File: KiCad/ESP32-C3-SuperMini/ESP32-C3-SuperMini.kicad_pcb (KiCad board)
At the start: 2 copper layers, 18 x 22.5 mm, 39 parts, among them J1 USB_C_Receptacle_USB2.0_14P, SW1 SW_Push, SW2 SW_Push, U1 ESP32-C3, U2 ME6211C33M5G, Y1 Crystal_GND24

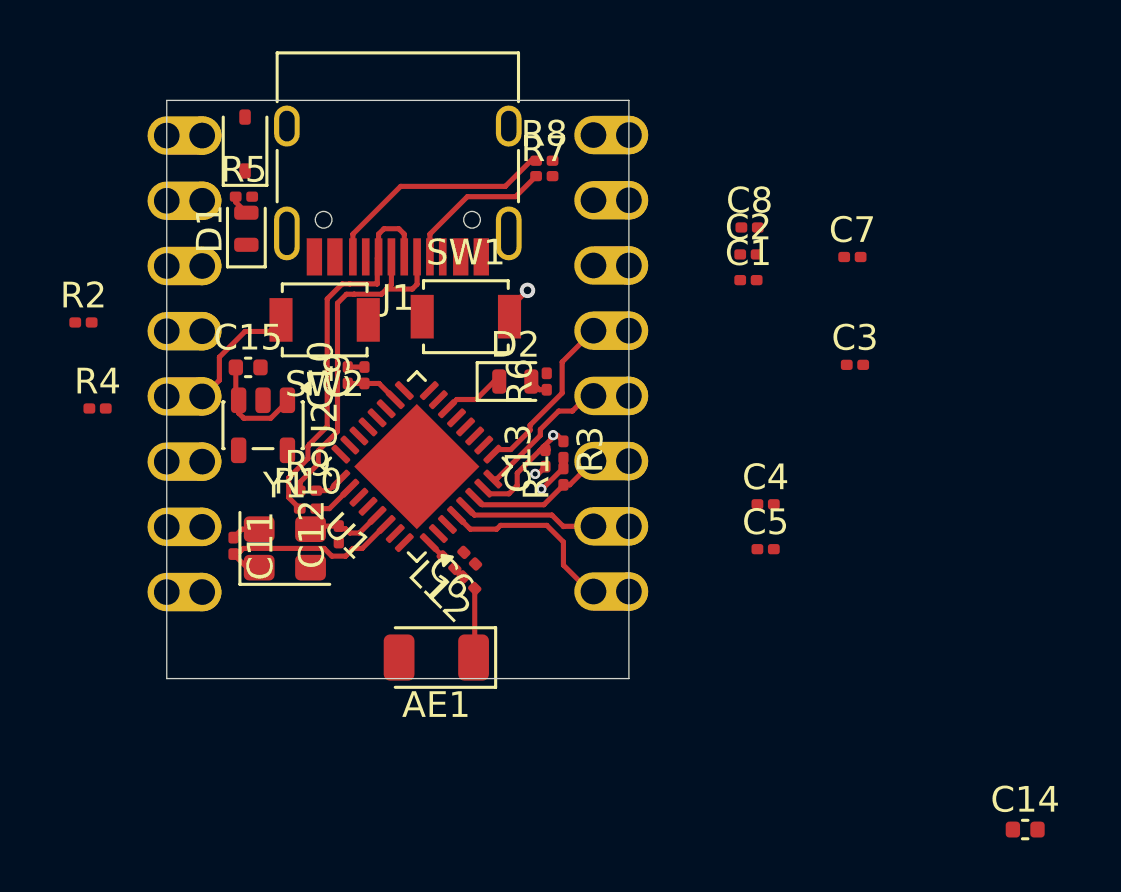
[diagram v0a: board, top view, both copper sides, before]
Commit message: wip
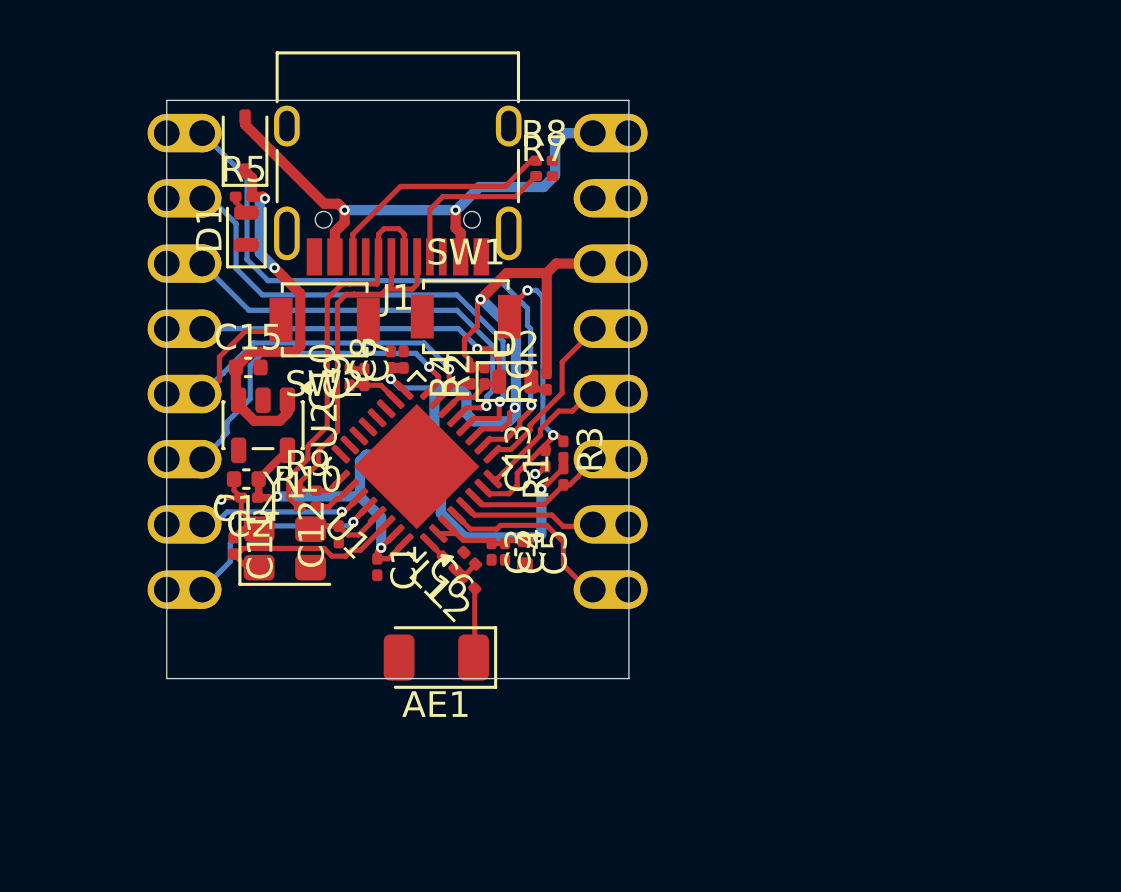
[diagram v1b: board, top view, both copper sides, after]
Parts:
- C5: footprint Capacitor_SMD:C_0201_0603Metric -> Capacitor_SMD:C_0402_1005Metric
- moved C14 33.3 mm to (45.1, 44.8), turned to 180 degrees
- moved C2 21.6 mm to (45.3, 45.5), turned to 180 degrees
- moved C1 18.3 mm to (50.2, 48.2), turned to -90 degrees
- moved C7 17.9 mm to (51.3, 40.1), turned to 90 degrees
- moved C3 15.9 mm to (54.7, 47.6), turned to -90 degrees
- moved R2 15.8 mm to (54.4, 40.7), turned to 90 degrees
- moved C8 14.9 mm to (50.8, 40.1), turned to 90 degrees
- moved R4 14.6 mm to (53.9, 40.7), turned to 90 degrees
- moved C4 10.3 mm to (55.2, 47.6), turned to -90 degrees
- moved C5 9.38 mm to (56.0, 47.6), turned to -90 degrees
- moved C10 0.10 mm to (49.2, 40.8)
- moved H1 0.10 mm to (42.0, 31.3)
- moved H2 0.08 mm to (58.6, 31.3)
- moved R10 0.07 mm to (47.5, 45.8)
- moved C9 0.07 mm to (49.8, 40.8)
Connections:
- D3 pad 2: Net-(D3-A) -> VBUS
- J1 pad A4: Net-(D3-A) -> VBUS
- J1 pad A9: Net-(D3-A) -> VBUS
- J1 pad B4: Net-(D3-A) -> VBUS
- J1 pad B9: Net-(D3-A) -> VBUS
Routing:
- net +3.3V: track 1.61 -> 60.3 mm, vias 1 -> 7
- net /GPIO5/ADC2/SCL: track 0.00 -> 23.9 mm, vias 0 -> 1
- net VBUS: track 0.00 -> 21.0 mm, vias 0 -> 2
- net /GPIO6: track 0.00 -> 19.7 mm, vias 0 -> 1
- net /GPIO7: track 0.00 -> 16.5 mm, vias 0 -> 1
- net /GPIO8/PWM: track 2.46 -> 15.7 mm, vias 0 -> 1
- net /GPIO9/BOOT: track 4.83 -> 18.0 mm, vias 0 -> 1
- net /GPIO10: track 0.00 -> 13.0 mm, vias 0 -> 1
- net /VSYS: track 4.24 -> 15.4 mm, vias 0 -> 2
- net /GPIO21: track 0.00 -> 8.26 mm, vias 0 -> 1
- net /GPIO20: track 0.00 -> 6.54 mm, vias 0 -> 1
- net /CHIP_EN: track 6.43 -> 12.7 mm
- net GND: track 2.31 -> 5.37 mm, vias 1 -> 2
- net Net-(C6-Pad1): track 0.46 -> 1.16 mm
- net Net-(J1-CC1): track 5.96 -> 6.52 mm
